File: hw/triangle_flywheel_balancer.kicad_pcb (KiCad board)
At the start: 4 copper layers, 40 x 30 mm, 0 parts

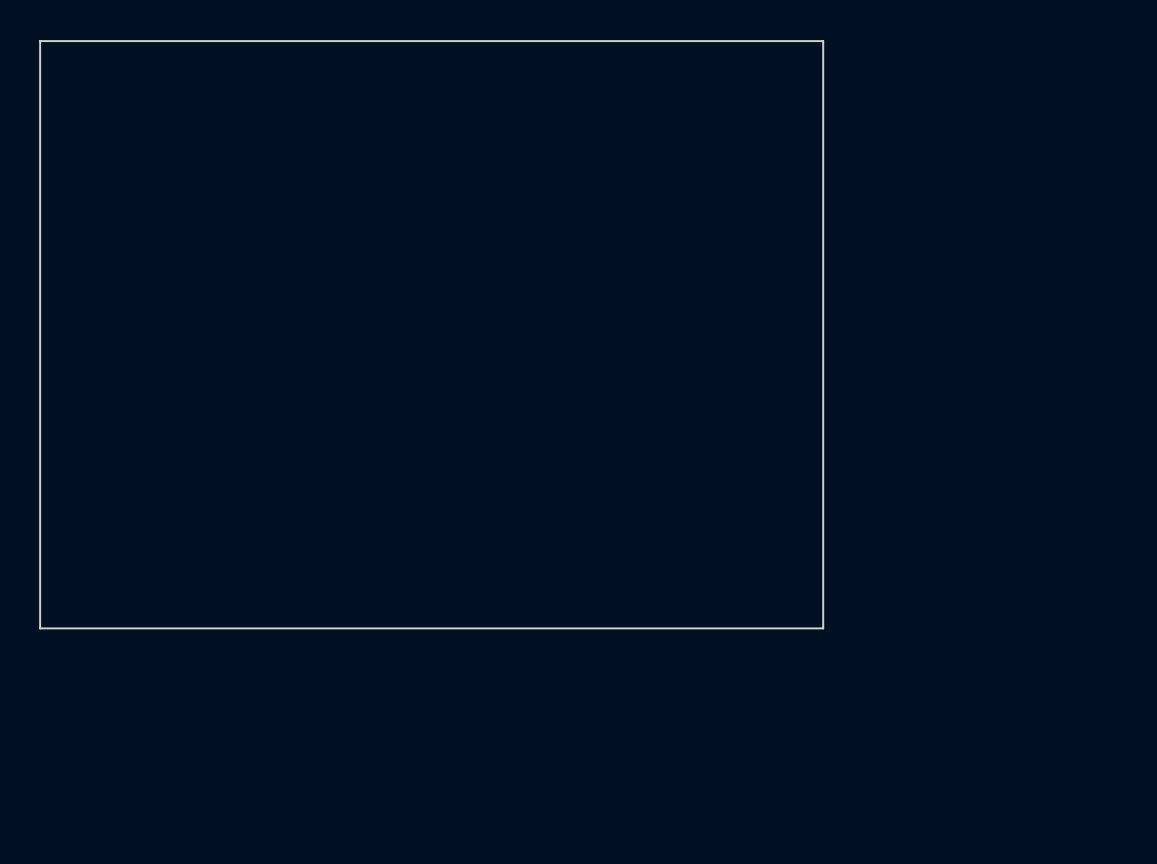
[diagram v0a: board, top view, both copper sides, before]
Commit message: Project init
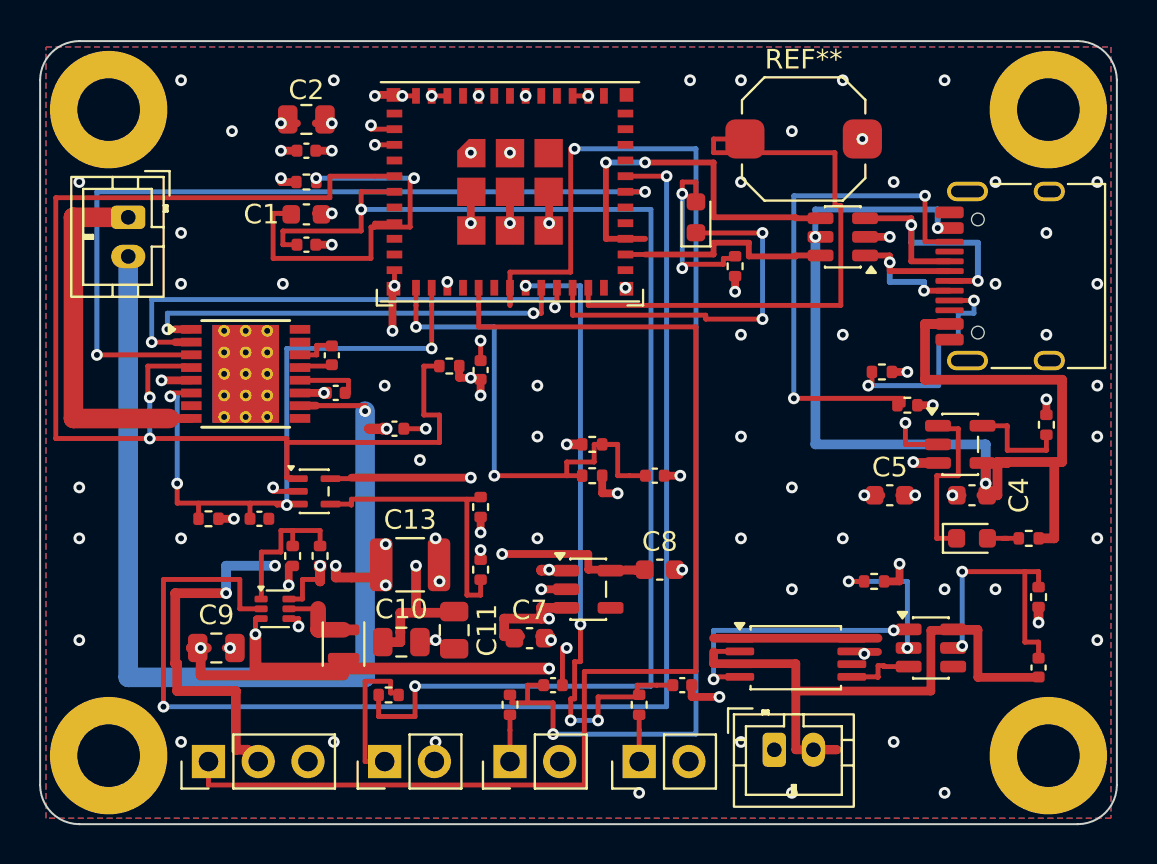
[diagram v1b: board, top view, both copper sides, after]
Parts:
- added C1: 1uF, triangle_flywheel_balancer:C_0603_1608Metric, F.Cu at (113.6, 108.8)
- added C10: 22uF, triangle_flywheel_balancer:C_0805_2012Metric, F.Cu at (118.5, 130.7)
- added C11: 22uF, triangle_flywheel_balancer:C_0805_2012Metric, F.Cu at (121.2, 130.1)
- added C12: 100nF, triangle_flywheel_balancer:C_0402_1005Metric, F.Cu at (118.1, 119.8)
- added C13: 100uF, triangle_flywheel_balancer:C_1210_3225Metric, F.Cu at (118.9, 126.8)
- added C14: 100nF, triangle_flywheel_balancer:C_0402_1005Metric, F.Cu at (115.1, 118.0)
- added C15: 22nF, triangle_flywheel_balancer:C_0402_1005Metric, F.Cu at (114.9, 116.0)
- added C16: 1nF, triangle_flywheel_balancer:C_0402_1005Metric, F.Cu at (111.2, 124.4)
- added C17: 100nF, triangle_flywheel_balancer:C_0402_1005Metric, F.Cu at (122.5, 116.8)
- added C18: 100nF, triangle_flywheel_balancer:C_0402_1005Metric, F.Cu at (131.4, 122.2)
- added C19: 100nF, triangle_flywheel_balancer:C_0402_1005Metric, F.Cu at (113.6, 110.4)
- added C2: 10uF, triangle_flywheel_balancer:C_0805_2012Metric, F.Cu at (113.6, 104.0)
- added C20: 100nF, triangle_flywheel_balancer:C_0402_1005Metric, F.Cu at (126.2, 132.9)
- added C21: 100nF, triangle_flywheel_balancer:C_0402_1005Metric, F.Cu at (132.8, 132.9)
- added C3: 100nF, triangle_flywheel_balancer:C_0402_1005Metric, F.Cu at (113.6, 105.6)
- added C4: 4.7uF, triangle_flywheel_balancer:C_0603_1608Metric, F.Cu at (147.6, 123.2)
- added C5: 4.7uF, triangle_flywheel_balancer:C_0603_1608Metric, F.Cu at (143.4, 123.2)
- added C6: 100nF, triangle_flywheel_balancer:C_0402_1005Metric, F.Cu at (151.0, 132.0)
- added C7: 1uF, triangle_flywheel_balancer:C_0603_1608Metric, F.Cu at (125.0, 130.5)
- added C8: 1uF, triangle_flywheel_balancer:C_0603_1608Metric, F.Cu at (131.7, 127.0)
- added C9: 10uF, triangle_flywheel_balancer:C_0805_2012Metric, F.Cu at (109.0, 131.0)
- added D1: USBLC6-2SC6, triangle_flywheel_balancer:SOT-23-6, F.Cu at (141.0, 110.0)
- added D2: LED, triangle_flywheel_balancer:LED_0603_1608Metric, F.Cu at (147.6, 125.4)
- added D3: LED, triangle_flywheel_balancer:LED_0603_1608Metric, F.Cu at (133.5, 109.0)
- added H1: MountingHole, triangle_flywheel_balancer:MountingHole_3.2mm_M2.5, F.Cu at (103.5, 103.5)
- added H2: MountingHole, triangle_flywheel_balancer:MountingHole_3.2mm_M2.5, F.Cu at (151.5, 103.5)
- added H3: MountingHole, triangle_flywheel_balancer:MountingHole_3.2mm_M2.5, F.Cu at (103.5, 136.5)
- added H4: MountingHole, triangle_flywheel_balancer:MountingHole_3.2mm_M2.5, F.Cu at (151.5, 136.5)
- added J1: TYPE-C-31-M-12, triangle_flywheel_balancer:USB_C_Receptacle_HRO_TYPE-C-31-M-12, F.Cu at (150.5, 112.0)
- added J2: BATTERY, triangle_flywheel_balancer:JST_PH_B2B-PH-K_1x02_P2.00mm_Vertical, F.Cu at (137.5, 136.2)
- added J3: MOTOR, triangle_flywheel_balancer:JST_PH_B2B-PH-K_1x02_P2.00mm_Vertical, F.Cu at (104.5, 109.0)
- added J4: SERVO, triangle_flywheel_balancer:PinHeader_1x03_P2.54mm_Vertical, F.Cu at (108.6, 136.8)
- added J5: LATCH, triangle_flywheel_balancer:PinHeader_1x02_P2.54mm_Vertical, F.Cu at (117.6, 136.8)
- added J6: OPEN, triangle_flywheel_balancer:PinHeader_1x02_P2.54mm_Vertical, F.Cu at (124.0, 136.8)
- added J7: CLOSED, triangle_flywheel_balancer:PinHeader_1x02_P2.54mm_Vertical, F.Cu at (130.6, 136.8)
- added L1: 1uH, triangle_flywheel_balancer:L_Murata_DFE201610P, F.Cu at (115.5, 130.8)
- added Q1: FS8205A, triangle_flywheel_balancer:TSSOP-8_4.4x3mm_P0.65mm, F.Cu at (138.6, 131.5)
- added R1: 10k, triangle_flywheel_balancer:R_0402_1005Metric, F.Cu at (113.6, 107.2)
- added R10: 1k, triangle_flywheel_balancer:R_0402_1005Metric, F.Cu at (108.6, 124.4)
- added R11: 33k, triangle_flywheel_balancer:R_0402_1005Metric, F.Cu at (122.5, 123.8)
- added R12: 51k, triangle_flywheel_balancer:R_0402_1005Metric, F.Cu at (122.5, 127.0)
- added R13: 100k, triangle_flywheel_balancer:R_0402_1005Metric, F.Cu at (120.9, 116.6)
- added R14: 1k, triangle_flywheel_balancer:R_0402_1005Metric, F.Cu at (135.5, 111.5)
- added R15: 100k, triangle_flywheel_balancer:R_0402_1005Metric, F.Cu at (128.2, 120.6)
- added R16: 100k, triangle_flywheel_balancer:R_0402_1005Metric, F.Cu at (128.2, 122.2)
- added R17: 1k, triangle_flywheel_balancer:R_0402_1005Metric, F.Cu at (117.8, 133.4)
- added R18: 1k, triangle_flywheel_balancer:R_0402_1005Metric, F.Cu at (124.0, 133.9)
- added R19: 1k, triangle_flywheel_balancer:R_0402_1005Metric, F.Cu at (130.6, 133.9)
- added R2: 5.1k, triangle_flywheel_balancer:R_0402_1005Metric, F.Cu at (143.0, 116.9)
- added R3: 5.1k, triangle_flywheel_balancer:R_0402_1005Metric, F.Cu at (144.3, 118.6)
- added R4: 1k, triangle_flywheel_balancer:R_0402_1005Metric, F.Cu at (150.5, 125.4)
- added R5: 2k, triangle_flywheel_balancer:R_0402_1005Metric, F.Cu at (151.4, 119.6)
- added R6: 330, triangle_flywheel_balancer:R_0402_1005Metric, F.Cu at (151.0, 128.4)
- added R7: 1k, triangle_flywheel_balancer:R_0402_1005Metric, F.Cu at (142.6, 127.6)
- added R8: 1.1M, triangle_flywheel_balancer:R_0402_1005Metric, F.Cu at (114.3, 126.3)
- added R9: 150k, triangle_flywheel_balancer:R_0402_1005Metric, F.Cu at (112.9, 126.3)
- added S4: SW_Push, triangle_flywheel_balancer:SW_Push_1TS009xxxx-xxxx-xxxx_6x6x5mm, F.Cu at (139.0, 105.0)
- added U1: ESP32-C3-MINI-1-N4, triangle_flywheel_balancer:ESP32-C3-MINI-1, F.Cu at (124.0, 105.0)
- added U2: DRV8876PWPR, triangle_flywheel_balancer:HTSSOP-16-1EP_4.4x5mm_P0.65mm_EP3.4x5mm_Mask3x3mm_ThermalVias, F.Cu at (110.5, 117.0)
- added U3: TLV7041DCKR, triangle_flywheel_balancer:SOT-353_SC-70-5, F.Cu at (114.0, 123.0)
- added U4: MCP73831T-2ACI/OT, triangle_flywheel_balancer:SOT-23-5, F.Cu at (147.0, 120.6)
- added U5: DW01A, triangle_flywheel_balancer:SOT-23-6, F.Cu at (145.5, 131.0)
- added U6: XC6220B331MR-G, triangle_flywheel_balancer:SOT-23-5, F.Cu at (128.0, 128.0)
- added U7: TPS61023DRLR, triangle_flywheel_balancer:SOT-563, F.Cu at (112.0, 129.0)
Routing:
- net BOOST_EN: track 0.00 -> 67.9 mm, vias 0 -> 2
- net SW_LATCH: track 0.00 -> 64.8 mm, vias 0 -> 2
- net nFAULT_ANY: track 0.00 -> 64.5 mm, vias 0 -> 2
- net SERVO_PWM: track 0.00 -> 62.6 mm
- net SW_OPEN: track 0.00 -> 61.5 mm, vias 0 -> 2
- net VBUS: track 0.00 -> 60.4 mm, vias 0 -> 3
- net MOTOR_B: track 0.00 -> 50.8 mm, vias 0 -> 1
- net GND: track 0.00 -> 44.6 mm, vias 0 -> 98
- net DRV_NSLEEP: track 0.00 -> 42.1 mm, vias 0 -> 2
- net VBAT: track 0.00 -> 40.1 mm, vias 0 -> 9
- net +5V: track 0.00 -> 37.7 mm, vias 0 -> 9
- net IPROPI: track 0.00 -> 35.0 mm, vias 0 -> 4
- net BATT_N: track 0.00 -> 34.5 mm
- net SW_CLOSED: track 0.00 -> 32.9 mm, vias 0 -> 4
- net BUTTON: track 0.00 -> 30.4 mm
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- added copper zone on In2.Cu, net +3V3
- added copper zone on In2.Cu, net +5V
- added copper zone on B.Cu, net GND
- added copper zone on F.Cu, net GND
- added copper zone on In1.Cu, net GND
- added copper zone on In2.Cu, net VBAT
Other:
- board size 40 x 30 mm -> 55 x 40 mm
